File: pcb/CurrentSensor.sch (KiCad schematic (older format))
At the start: 4 parts, among them U5 ACS711

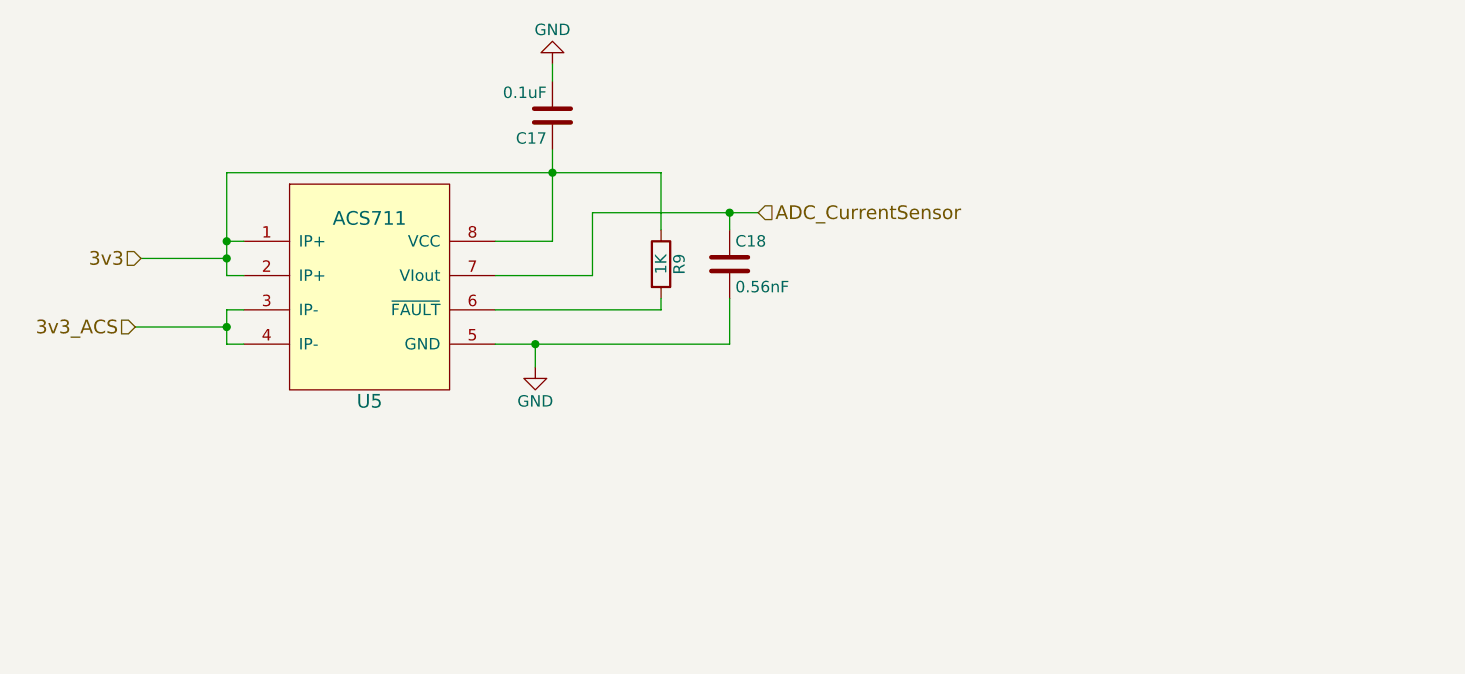
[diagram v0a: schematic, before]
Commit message: Clean up Kicad and TCC
Some changes in the
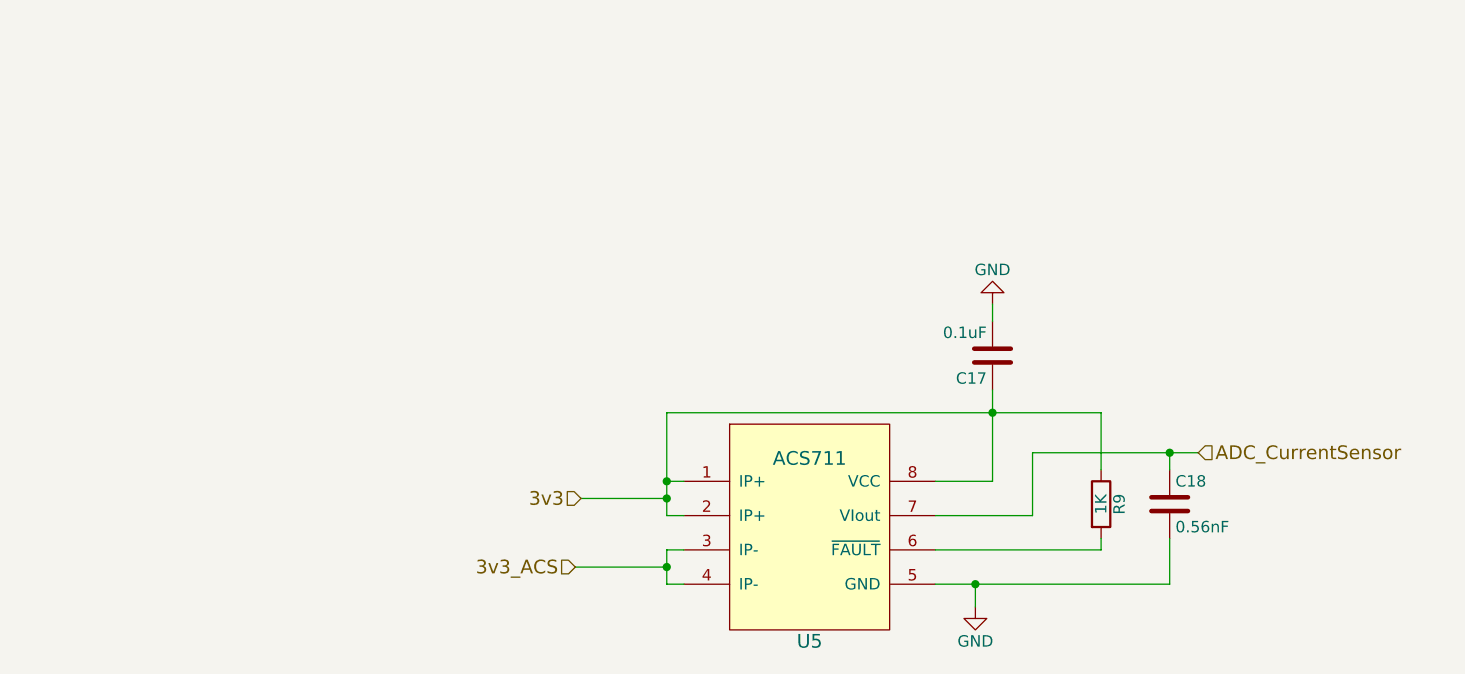
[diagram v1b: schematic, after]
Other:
- moved on the sheet: C17, C18, R9, U5
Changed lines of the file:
@@
 encoding utf-8
 Sheet 5 10
-Title ""
+Title "Current Sensor Schematic"
 Date ""
-Rev ""
-Comp ""
+Rev "1"
+Comp "Universidade de Brasília - Campus Gama"
 Comment1 ""
 Comment2 ""
@@
 L power:GND #PWR08
 U 1 1 5B5D63DB
-P 4575 3175
-F 0 "#PWR08" H 4575 2925 50  0001 C CNN
-F 1 "GND" H 4575 3025 50  0000 C CNN
-F 2 "" H 4575 3175 50  0001 C CNN
-F 3 "" H 4575 3175 50  0001 C CNN
-	1    4575 3175
+P 6500 4225
+F 0 "#PWR08" H 6500 3975 50  0001 C CNN
+F 1 "GND" H 6500 4075 50  0000 C CNN
+F 2 "" H 6500 4225 50  0001 C CNN
+F 3 "" H 6500 4225 50  0001 C CNN
+	1    6500 4225
 	1    0    0    -1
 $EndComp
-Text HLabel 2850 2700 0    60   Input ~ 0
+Text HLabel 4775 3750 0    60   Input ~ 0
 3v3
-Text HLabel 5550 2500 2    60   Input ~ 0
+Text HLabel 7475 3550 2    60   Input ~ 0
 ADC_CurrentSensor
-Text HLabel 2825 3000 0    60   Input ~ 0
+Text HLabel 4750 4050 0    60   Input ~ 0
 3v3_ACS
 $Comp
 L Device:C C17
 U 1 1 5B5DC977
-P 4650 2075
-F 0 "C17" H 4675 2175 50  0000 L CNN
-F 1 "0.1uF" H 4675 1975 50  0000 L CNN
-F 2 "Capacitors_SMD:C_1206" H 4688 1925 50  0001 C CNN
-F 3 "https://www.digikey.com/product-detail/en/yageo/CC1206KRX7R9BB104/311-1179-1-ND/303089" H 4650 2075 50  0001 C CNN
-	1    4650 2075
+P 6575 3125
+F 0 "C17" H 6600 3225 50  0000 L CNN
+F 1 "0.1uF" H 6600 3025 50  0000 L CNN
+F 2 "Capacitors_SMD:C_1206" H 6613 2975 50  0001 C CNN
+F 3 "https://www.digikey.com/product-detail/en/yageo/CC1206KRX7R9BB104/311-1179-1-ND/303089" H 6575 3125 50  0001 C CNN
+	1    6575 3125
 	-1   0    0    1
 $EndComp
@@
 L acs711:ACS711 U5
 U 1 1 5B5DD146
-P 3850 3325
-F 0 "U5" H 3850 3325 60  0000 C CNN
-F 1 "ACS711" H 3850 4125 60  0000 C CNN
-F 2 ".pretty:ACS711_8-pin SOICN" H 3850 3325 60  0001 C CNN
-F 3 "https://www.digikey.com/product-detail/en/allegro-microsystems-llc/ACS711ELCTR-12AB-T/620-1370-1-ND/2470594" H 3850 3325 60  0001 C CNN
-	1    3850 3325
+P 5775 4375
+F 0 "U5" H 5775 4375 60  0000 C CNN
+F 1 "ACS711" H 5775 5175 60  0000 C CNN
+F 2 ".pretty:ACS711_8-pin SOICN" H 5775 4375 60  0001 C CNN
+F 3 "https://www.digikey.com/product-detail/en/allegro-microsystems-llc/ACS711ELCTR-12AB-T/620-1370-1-ND/2470594" H 5775 4375 60  0001 C CNN
+	1    5775 4375
 	1    0    0    -1
 $EndComp
 Wire Wire Line
-	3300 2925 3225 2925
+	5225 3975 5150 3975
 Wire Wire Line
-	3225 2925 3225 3000
+	5150 3975 5150 4050
 Wire Wire Line
-	3225 3075 3300 3075
+	5150 4125 5225 4125
 Wire Wire Line
-	2825 3000 3225 3000
-Connection ~ 3225 3000
+	4750 4050 5150 4050
+Connection ~ 5150 4050
 Wire Wire Line
-	4400 3075 4575 3075
+	6325 4125 6500 4125
 Wire Wire Line
-	4575 3075 4575 3175
+	6500 4125 6500 4225
 Wire Wire Line
-	4650 2625 4400 2625
+	6575 3675 6325 3675
 Wire Wire Line
-	4650 2225 4650 2325
+	6575 3275 6575 3375
 Wire Wire Line
-	3225 2325 4650 2325
-Connection ~ 4650 2325
+	5150 3375 6575 3375
+Connection ~ 6575 3375
 $Comp
 L power:GND #PWR09
 U 1 1 5B5DD45F
-P 4650 1850
-F 0 "#PWR09" H 4650 1600 50  0001 C CNN
-F 1 "GND" H 4650 1700 50  0000 C CNN
-F 2 "" H 4650 1850 50  0001 C CNN
-F 3 "" H 4650 1850 50  0001 C CNN
-	1    4650 1850
+P 6575 2900
+F 0 "#PWR09" H 6575 2650 50  0001 C CNN
+F 1 "GND" H 6575 2750 50  0000 C CNN
+F 2 "" H 6575 2900 50  0001 C CNN
+F 3 "" H 6575 2900 50  0001 C CNN
+	1    6575 2900
 	-1   0    0    1
 $EndComp
 Wire Wire Line
-	4650 1850 4650 1925
+	6575 2900 6575 2975
 $Comp
 L Device:R R9
 U 1 1 5B5DD491
-P 5125 2725
-F 0 "R9" V 5205 2725 50  0000 C CNN
-F 1 "1K" V 5125 2725 50  0000 C CNN
-F 2 "Resistors_SMD:R_1206" V 5055 2725 50  0001 C CNN
-F 3 "https://www.digikey.com/product-detail/en/stackpole-electronics-inc/RNCP1206FTD1K00/RNCP1206FTD1K00CT-ND/2240675" H 5125 2725 50  0001 C CNN
-	1    5125 2725
+P 7050 3775
+F 0 "R9" V 7130 3775 50  0000 C CNN
+F 1 "1K" V 7050 3775 50  0000 C CNN
+F 2 "Resistors_SMD:R_1206" V 6980 3775 50  0001 C CNN
+F 3 "https://www.digikey.com/product-detail/en/stackpole-electronics-inc/RNCP1206FTD1K00/RNCP1206FTD1K00CT-ND/2240675" H 7050 3775 50  0001 C CNN
+	1    7050 3775
 	1    0    0    -1
 $EndComp
 Wire Wire Line
-	5125 2875 5125 2925
+	7050 3925 7050 3975
 Wire Wire Line
-	5125 2925 4400 2925
+	7050 3975 6325 3975
 Wire Wire Line
-	5125 2325 5125 2575
+	7050 3375 7050 3625
 Wire Wire Line
-	4825 2500 5425 2500
+	6750 3550 7350 3550
 Wire Wire Line
-	4825 2500 4825 2775
+	6750 3550 6750 3825
 Wire Wire Line
-	4825 2775 4400 2775
+	6750 3825 6325 3825
 $Comp
 L Device:C C18
 U 1 1 5B5DD57D
-P 5425 2725
-F 0 "C18" H 5450 2825 50  0000 L CNN
-F 1 "0.56nF" H 5450 2625 50  0000 L CNN
-F 2 "Capacitors_SMD:C_1206" H 5463 2575 50  0001 C CNN
-F 3 "https://www.digikey.com/product-detail/en/kemet/C1206C511J5GAC7800/399-17482-1-ND/8570449" H 5425 2725 50  0001 C CNN
-	1    5425 2725
+P 7350 3775
+F 0 "C18" H 7375 3875 50  0000 L CNN
+F 1 "0.56nF" H 7375 3675 50  0000 L CNN
+F 2 "Capacitors_SMD:C_1206" H 7388 3625 50  0001 C CNN
+F 3 "https://www.digikey.com/product-detail/en/kemet/C1206C511J5GAC7800/399-17482-1-ND/8570449" H 7350 3775 50  0001 C CNN
+	1    7350 3775
 	1    0    0    -1
 $EndComp
 Wire Wire Line
-	5425 2575 5425 2500
-Connection ~ 5425 2500
+	7350 3625 7350 3550
+Connection ~ 7350 3550
 Wire Wire Line
-	5425 3075 5425 2875
-Connection ~ 4575 3075
+	7350 4125 7350 3925
+Connection ~ 6500 4125
 Wire Wire Line
-	3225 3000 3225 3075
+	5150 4050 5150 4125
 Wire Wire Line
-	4650 2325 4650 2625
+	6575 3375 6575 3675
 Wire Wire Line
-	4650 2325 5125 2325
+	6575 3375 7050 3375
 Wire Wire Line
-	5425 2500 5550 2500
+	7350 3550 7475 3550
 Wire Wire Line
-	4575 3075 5425 3075
+	6500 4125 7350 4125
 Wire Wire Line
-	3225 2325 3225 2625
+	5150 3375 5150 3675
 Wire Wire Line
-	3300 2625 3225 2625
-Connection ~ 3225 2625
+	5225 3675 5150 3675
+Connection ~ 5150 3675
 Wire Wire Line
-	3225 2625 3225 2700
+	5150 3675 5150 3750
 Wire Wire Line
-	3300 2775 3225 2775
+	5225 3825 5150 3825
 Wire Wire Line
-	2850 2700 3225 2700
-Connection ~ 3225 2700
+	4775 3750 5150 3750
+Connection ~ 5150 3750
 Wire Wire Line
-	3225 2700 3225 2775
+	5150 3750 5150 3825
 $EndSCHEMATC
